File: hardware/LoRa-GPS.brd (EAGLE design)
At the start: 50.8 x 17.8 mm, 26 parts, among them J2 MF-CON-MICROUSB-RIGHT, U1 MCP1703-3302E/CB, Y1 CRYSTAL.ABS07

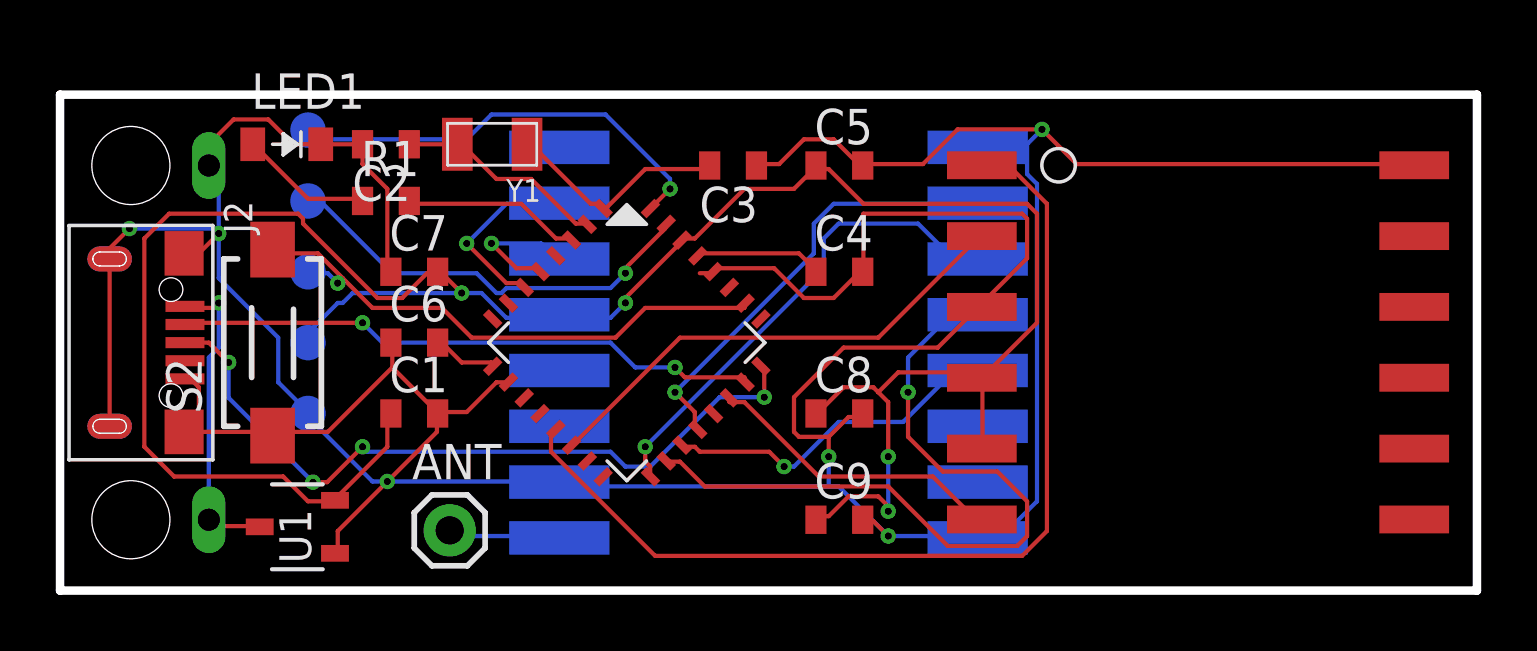
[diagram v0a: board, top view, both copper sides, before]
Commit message: tidy
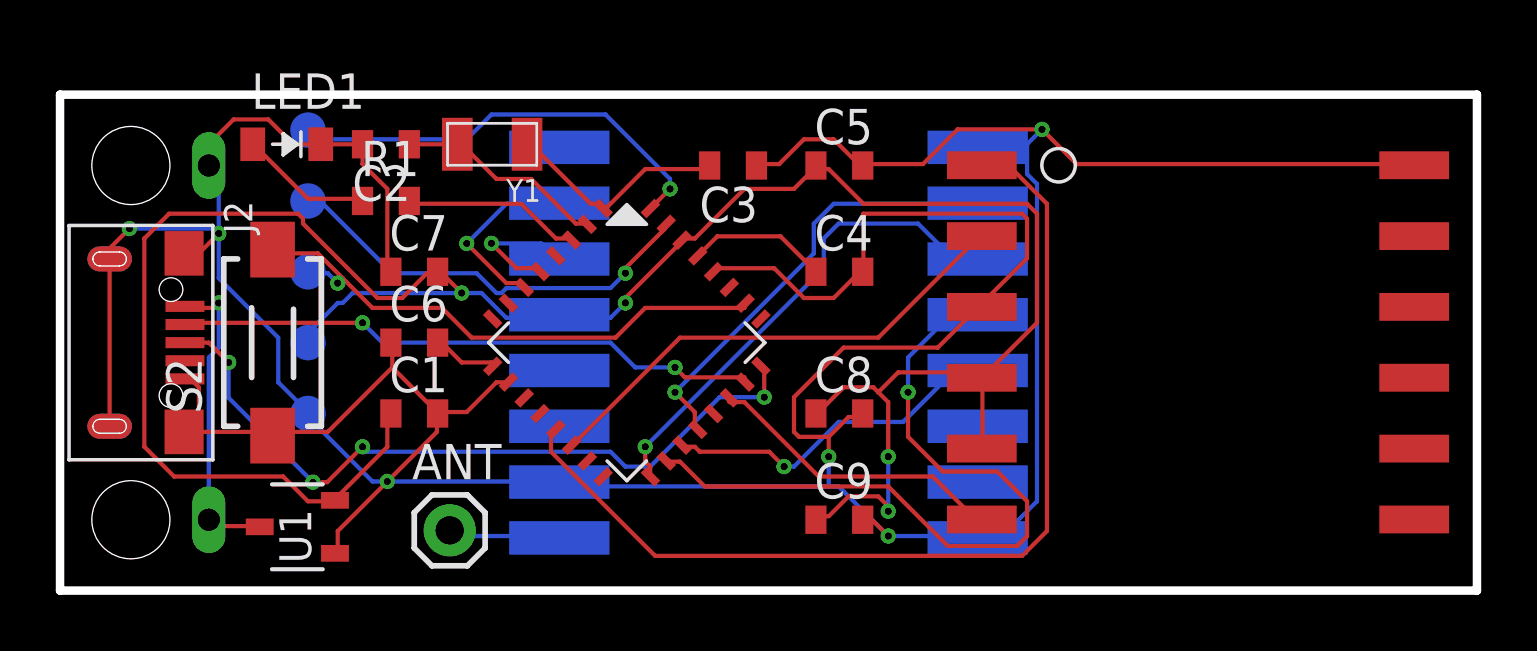
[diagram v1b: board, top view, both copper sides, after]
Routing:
- net GND: track 164.7 -> 164.0 mm
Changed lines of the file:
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@@
 <drawing>
 <settings>
-<setting alwaysvectorfont="yes"/>
+<setting alwaysvectorfont="no"/>
 <setting keepoldvectorfont="yes"/>
 <setting verticaltext="up"/>
@@
 <layer number="23" name="tOrigins" color="15" fill="1" visible="yes" active="yes"/>
 <layer number="24" name="bOrigins" color="15" fill="1" visible="yes" active="yes"/>
-<layer number="25" name="tNames" color="7" fill="1" visible="yes" active="yes"/>
-<layer number="26" name="bNames" color="7" fill="1" visible="yes" active="yes"/>
+<layer number="25" name="tNames" color="7" fill="1" visible="no" active="yes"/>
+<layer number="26" name="bNames" color="7" fill="1" visible="no" active="yes"/>
 <layer number="27" name="tValues" color="7" fill="1" visible="no" active="yes"/>
 <layer number="28" name="bValues" color="7" fill="1" visible="no" active="yes"/>
@@
 <layer number="37" name="tTest" color="7" fill="1" visible="no" active="yes"/>
 <layer number="38" name="bTest" color="7" fill="1" visible="no" active="yes"/>
-<layer number="39" name="tKeepout" color="4" fill="11" visible="yes" active="yes"/>
-<layer number="40" name="bKeepout" color="1" fill="11" visible="yes" active="yes"/>
-<layer number="41" name="tRestrict" color="4" fill="10" visible="yes" active="yes"/>
-<layer number="42" name="bRestrict" color="1" fill="10" visible="yes" active="yes"/>
+<layer number="39" name="tKeepout" color="4" fill="11" visible="no" active="yes"/>
+<layer number="40" name="bKeepout" color="1" fill="11" visible="no" active="yes"/>
+<layer number="41" name="tRestrict" color="4" fill="10" visible="no" active="yes"/>
+<layer number="42" name="bRestrict" color="1" fill="10" visible="no" active="yes"/>
 <layer number="43" name="vRestrict" color="2" fill="10" visible="no" active="yes"/>
 <layer number="44" name="Drills" color="7" fill="1" visible="no" active="yes"/>
-<layer number="45" name="Holes" color="7" fill="1" visible="no" active="yes"/>
+<layer number="45" name="Holes" color="7" fill="1" visible="yes" active="yes"/>
 <layer number="46" name="Milling" color="3" fill="1" visible="no" active="yes"/>
 <layer number="47" name="Measures" color="7" fill="1" visible="no" active="yes"/>
@@
 <layer number="50" name="dxf" color="7" fill="1" visible="no" active="no"/>
 <layer number="51" name="tDocu" color="6" fill="1" visible="yes" active="yes"/>
-<layer number="52" name="bDocu" color="7" fill="1" visible="yes" active="yes"/>
+<layer number="52" name="bDocu" color="7" fill="1" visible="no" active="yes"/>
 <layer number="53" name="tGND_GNDA" color="7" fill="9" visible="no" active="no"/>
 <layer number="54" name="bGND_GNDA" color="1" fill="9" visible="no" active="no"/>
@@
 <contactref element="C1" pad="2"/>
 <contactref element="C4" pad="2"/>
-<contactref element="SAMD21" pad="28"/>
 <contactref element="C5" pad="2"/>
 <contactref element="J2" pad="5"/>
@@
 <wire x1="27.7368" y1="10.4902" x2="26.67" y2="10.4902" width="0.1524" layer="1"/>
 <wire x1="28.6258" y1="11.3792" x2="27.7368" y2="10.4902" width="0.1524" layer="1"/>
-<wire x1="23.4696" y1="11.557" x2="23.43126875" y2="11.435584375" width="0.1524" layer="1"/>
 <wire x1="28.6258" y1="11.3792" x2="28.7782" y2="11.43" width="0.1524" layer="1"/>
 <wire x1="28.8036" y1="11.557" x2="28.8036" y2="13.5128" width="0.1524" layer="1"/>
@@
 <wire x1="9.779" y1="1.4224" x2="9.859" y2="1.336" width="0.1524" layer="1"/>
 <wire x1="7.6454" y1="5.5118" x2="7.62" y2="5.555" width="0.1524" layer="1"/>
-<wire x1="22.9362" y1="11.3792" x2="23.2918" y2="11.3792" width="0.1524" layer="1"/>
-<wire x1="23.2918" y1="11.3792" x2="23.43126875" y2="11.435584375" width="0.1524" layer="1"/>
 <wire x1="16.1798" y1="7.6454" x2="16.07735625" y2="7.475784375" width="0.1524" layer="1"/>
 <wire x1="34.671" y1="11.9126" x2="33.0708" y2="10.3124" width="0.1524" layer="1"/>
@@
 <vertex x="50.8" y="17.78"/>
 </polygon>
+<contactref element="SAMD21" pad="28"/>
 </signal>
 <signal name="VCC">
 <contactref element="C1" pad="1"/>
 <contactref element="U1" pad="2"/>
-<contactref element="SAMD21" pad="30"/>
 <contactref element="C5" pad="1"/>
 <contactref element="RADIO" pad="B4"/>
@@
 <wire x1="26.3144" y1="14.4018" x2="24.5364" y2="14.4018" width="0.1524" layer="1"/>
 <wire x1="27.0256" y1="15.113" x2="26.3144" y2="14.4018" width="0.1524" layer="1"/>
-<wire x1="22.4028" y1="12.6238" x2="22.299896875" y2="12.566953125" width="0.1524" layer="1"/>
 <wire x1="27.0256" y1="15.113" x2="27.1018" y2="15.24" width="0.1524" layer="1"/>
 <wire x1="27.559" y1="2.667" x2="27.2034" y2="2.667" width="0.1524" layer="1"/>
@@
 <wire x1="19.7358" y1="9.779" x2="20.2692" y2="10.3124" width="0.1524" layer="16"/>
 <wire x1="17.9578" y1="9.779" x2="19.7358" y2="9.779" width="0.1524" layer="16"/>
-<wire x1="22.225" y1="12.446" x2="22.299896875" y2="12.566953125" width="0.1524" layer="1"/>
 <wire x1="17.9578" y1="9.779" x2="17.9" y2="9.89" width="0.1524" layer="16"/>
 <via x="29.6926" y="2.8448" extent="1-16" drill="0.254"/>
@@
 <via x="14.4018" y="10.668" extent="1-16" drill="0.254"/>
 <via x="20.2692" y="10.3124" extent="1-16" drill="0.254"/>
-</signal>
-<signal name="N$5">
-<contactref element="SAMD21" pad="29"/>
-<contactref element="C4" pad="1"/>
-<wire x1="26.4922" y1="12.0904" x2="22.9362" y2="12.0904" width="0.1524" layer="1"/>
-<wire x1="27.0256" y1="11.557" x2="26.4922" y2="12.0904" width="0.1524" layer="1"/>
-<wire x1="22.9362" y1="12.0904" x2="22.865584375" y2="12.00126875" width="0.1524" layer="1"/>
-<wire x1="27.0256" y1="11.557" x2="27.1018" y2="11.43" width="0.1524" layer="1"/>
+<contactref element="SAMD21" pad="30"/>
+<wire x1="22.4028" y1="12.6238" x2="22.299896875" y2="12.566953125" width="0.1524" layer="1"/>
+<wire x1="22.225" y1="12.446" x2="22.299896875" y2="12.566953125" width="0.1524" layer="1"/>
 </signal>
 <signal name="VIN">
@@
 <signal name="N$10">
 </signal>
+<signal name="N$5">
+<contactref element="SAMD21" pad="29"/>
+<contactref element="C4" pad="1"/>
+<wire x1="22.865584375" y1="12.00126875" x2="23.564315625" y2="12.7" width="0.1524" layer="1"/>
+<wire x1="25.8318" y1="12.7" x2="27.1018" y2="11.43" width="0.1524" layer="1"/>
+<wire x1="23.564315625" y1="12.7" x2="25.8318" y2="12.7" width="0.1524" layer="1"/>
+</signal>
 </signals>
